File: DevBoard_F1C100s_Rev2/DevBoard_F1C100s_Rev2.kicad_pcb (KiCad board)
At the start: 2 copper layers, 46.5 x 75.8 mm, 92 parts, among them J1 LCD_40pin_FPC, J2 Micro_SD_Card_Det1, J3 USB_C_Receptacle_USB2.0_16P, SW1 RESET, SW2 RESET, SW3 FEL, U1 F1C100S, U2 W25Q16JVSS, U3 AP3031KTR-G1, U4 USBLC6-2SC6, U5 TPS562201DDCT, U6 TPS562201DDCT, U7 TPS562201DDCT, Y1 24Mhz

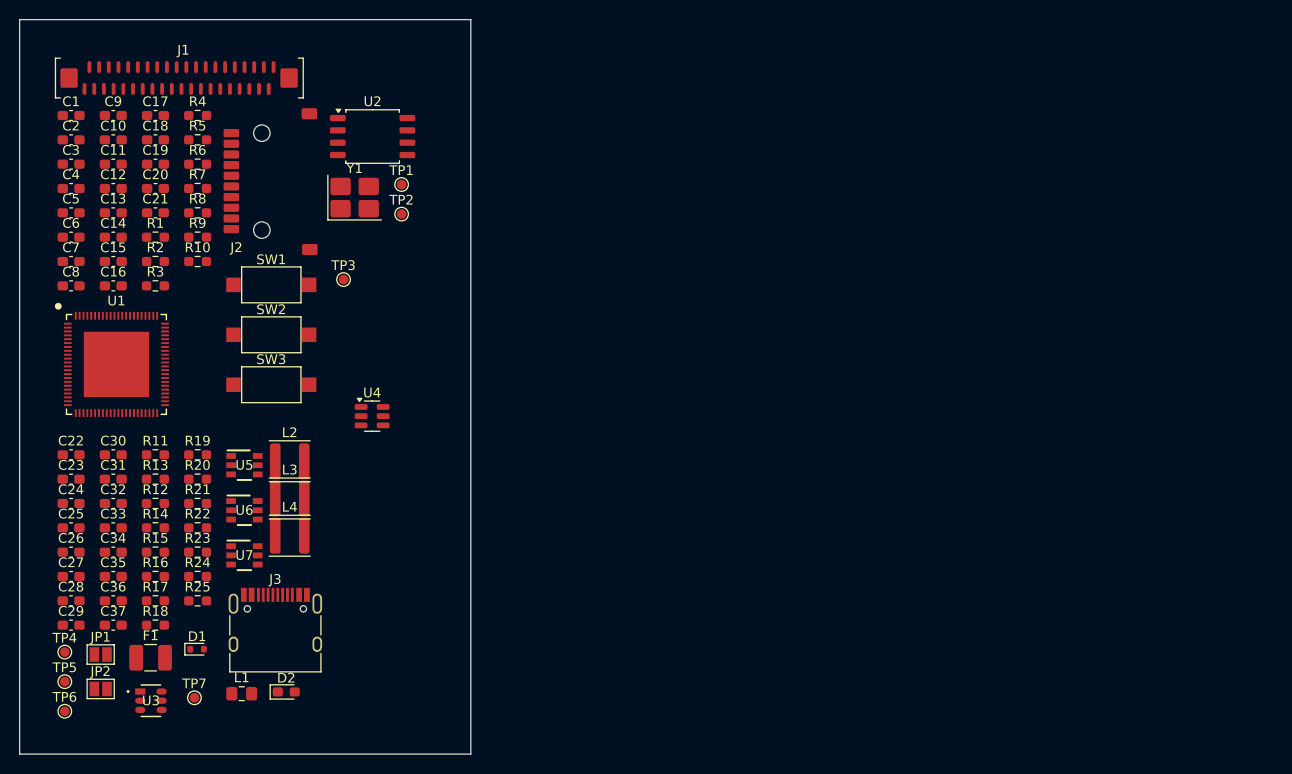
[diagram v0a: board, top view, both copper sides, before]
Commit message: Finish layout
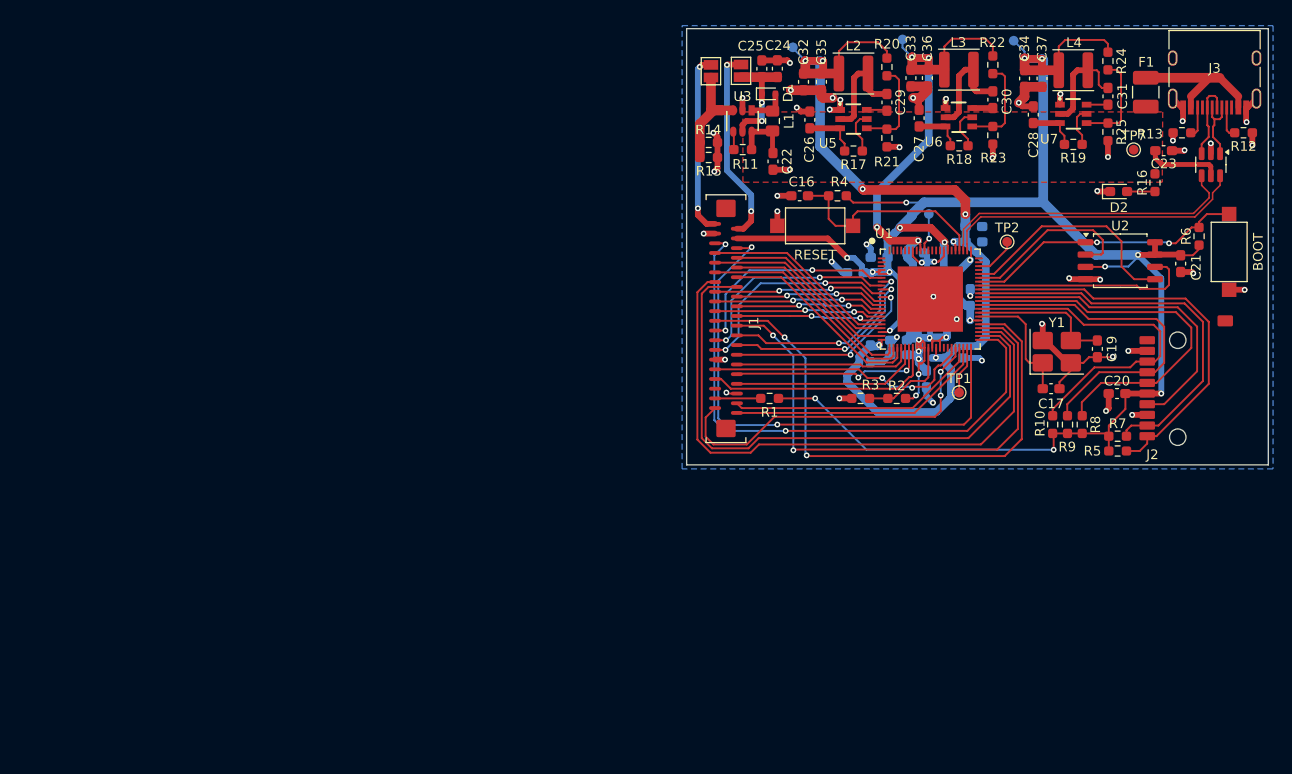
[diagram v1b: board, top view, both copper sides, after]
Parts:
- removed C1: 0.1uf, Capacitor_SMD:C_0603_1608Metric_Pad1.08x0.95mm_HandSolder
- removed SW1: RESET, Button_Switch_SMD:SW_SPST_CK_RS282G05A3
- C10, C11, C12, C13, C14, C15, C18, C2, C3, C4, C5, C6, C7, C8, C9, TP3, TP4, TP5, TP6: moved to B.Cu
- SW3: value FEL -> BOOT
- moved TP6 119.8 mm to (162.5, 33.3)
- moved R12 118.6 mm to (186.2, 42.8)
- moved F1 118.1 mm to (176.1, 38.6), turned to 90 degrees
- moved C23 117.7 mm to (177.9, 44.6)
- moved J3 113.1 mm to (183.2, 36.1), turned to 180 degrees
- moved TP7 112.2 mm to (174.8, 44.5)
- moved R13 111.7 mm to (179.8, 42.8), turned to 180 degrees
- moved C28 111.2 mm to (164.5, 40.9), turned to 90 degrees
- moved C37 111.2 mm to (165.4, 37.2), turned to -90 degrees
- moved R16 110.8 mm to (177.1, 48.0), turned to -90 degrees
- moved C31 109.9 mm to (172.2, 39.0), turned to 90 degrees
- moved TP5 108.9 mm to (151.0, 33.2)
- moved R24 107.9 mm to (172.2, 35.4), turned to -90 degrees
- moved C34 105.9 mm to (163.6, 37.2), turned to -90 degrees
- moved C21 105.9 mm to (179.7, 56.3), turned to -90 degrees
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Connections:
- net /LCD_RESET renamed Net-(J1-RESET)
- net Net-(F1-Pad2) renamed /Power/VBUS
- C19 pad 1: Net-(C19-Pad1) -> GND
- Y1 pad 2: Net-(C19-Pad1) -> GND
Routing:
- net 3.3V: track 0.00 -> 202.5 mm, vias 0 -> 16
- net GND: track 0.00 -> 107.4 mm, vias 0 -> 49
- net 1.1V: track 0.00 -> 94.5 mm, vias 0 -> 7
- net 2.6V: track 0.00 -> 87.6 mm, vias 0 -> 11
- net /LCD_D8: track 0.00 -> 63.5 mm
- net /LCD_D9: track 0.00 -> 62.1 mm
- net /LCD_D16: track 0.00 -> 59.7 mm, vias 0 -> 2
- net /LCD_D0: track 0.00 -> 59.3 mm, vias 0 -> 2
- net /LCD_D17: track 0.00 -> 54.5 mm, vias 0 -> 2
- net /LCD_D1: track 0.00 -> 54.5 mm, vias 0 -> 2
- net /SDC0_D1: track 0.00 -> 43.3 mm
- net /SDC0_D0: track 0.00 -> 41.0 mm
- net /SDC0_CMD: track 0.00 -> 40.1 mm
- net /SDC0_D3: track 0.00 -> 36.7 mm
- net /SPI1_CLK: track 0.00 -> 36.5 mm, vias 0 -> 2
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- added copper zone on F.Cu, net 5V
- added copper zone on B.Cu, net GND
- added copper zone on In1.Cu, net GND
- added copper zone on In2.Cu, net GND
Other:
- board size 46.5 x 75.8 mm -> 60 x 45 mm
- copper layers 2 -> 4
